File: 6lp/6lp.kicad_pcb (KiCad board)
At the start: 2 copper layers, 25.4 x 27.9 mm, 34 parts, among them J1 MODULE_HEADER, T1 2450BM15A0015, U1 AT86RF233, X1 16.0000MF09Z-AC3

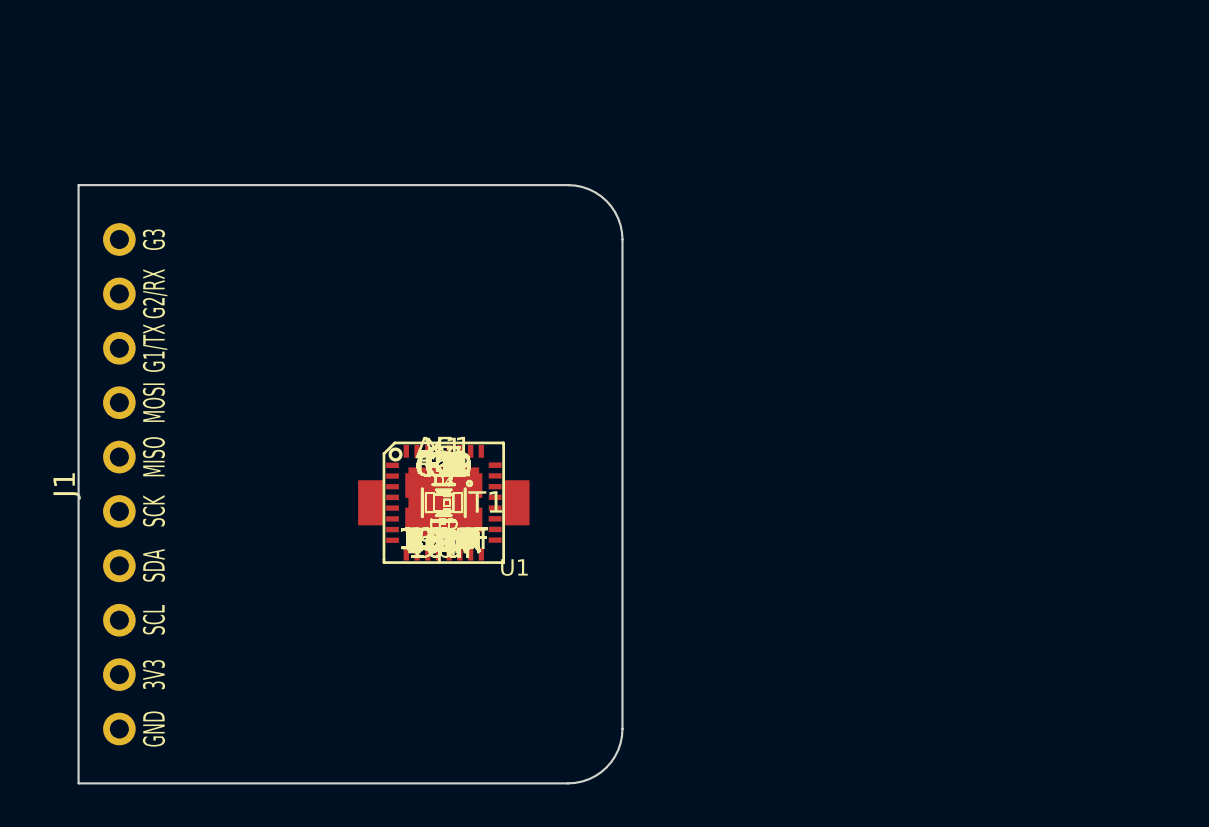
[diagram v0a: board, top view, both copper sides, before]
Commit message: invisible values
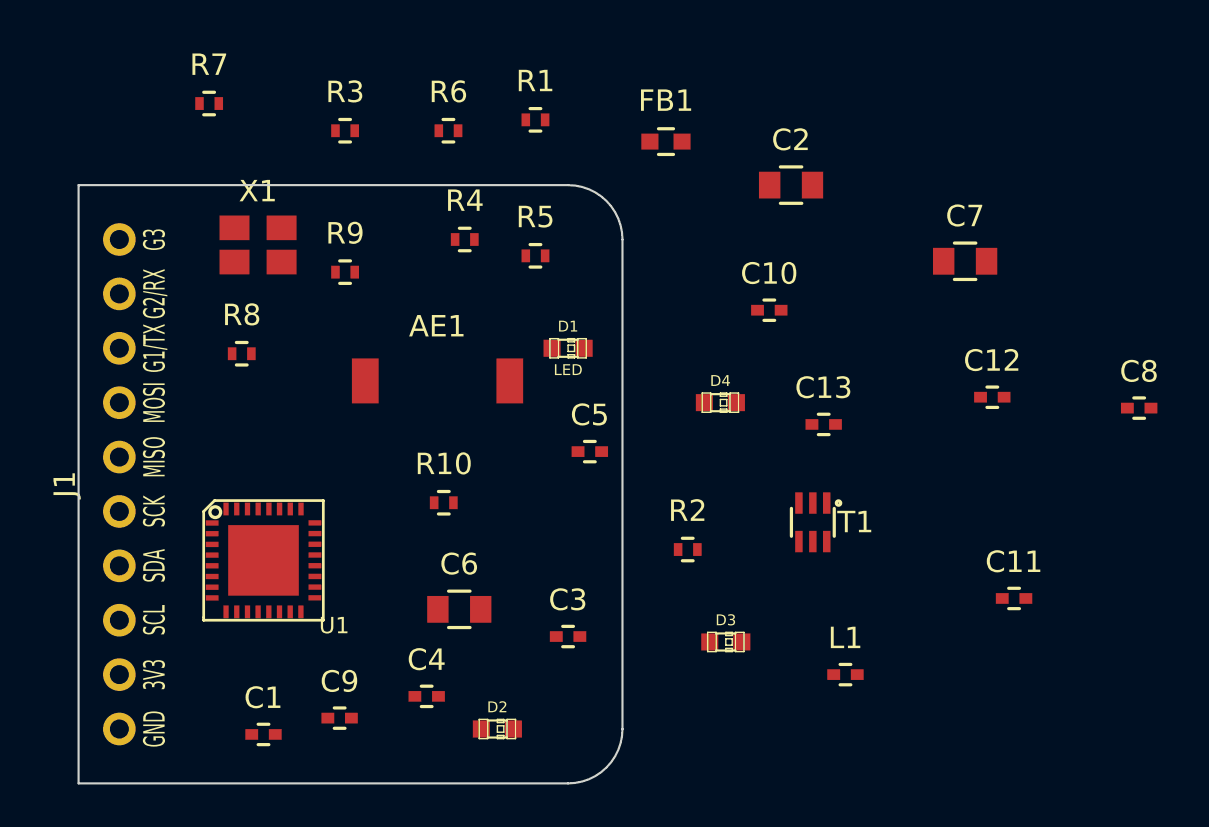
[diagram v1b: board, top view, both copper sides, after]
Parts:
- moved C8 32.8 mm to (176.5, 109.5)
- moved C11 27.0 mm to (170.7, 118.4)
- moved C7 26.8 mm to (168.4, 102.6)
- moved C12 26.1 mm to (169.7, 109.0)
- moved C2 22.0 mm to (160.3, 99.1)
- moved R7 21.6 mm to (133.1, 95.2)
- moved L1 20.4 mm to (162.8, 121.9)
- moved FB1 19.8 mm to (154.4, 97.0)
- moved R1 18.4 mm to (148.3, 96.0)
- moved C13 18.1 mm to (161.8, 110.2)
- moved R3 18.0 mm to (139.4, 96.5)
- moved C10 17.7 mm to (159.3, 104.9)
- moved R6 17.4 mm to (144.3, 96.5)
- moved T1 17.3 mm to (161.3, 114.8)
- moved X1 14.8 mm to (135.4, 101.9)
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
